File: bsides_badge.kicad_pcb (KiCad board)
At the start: 2 copper layers, 100.5 x 100.5 mm, 2 parts

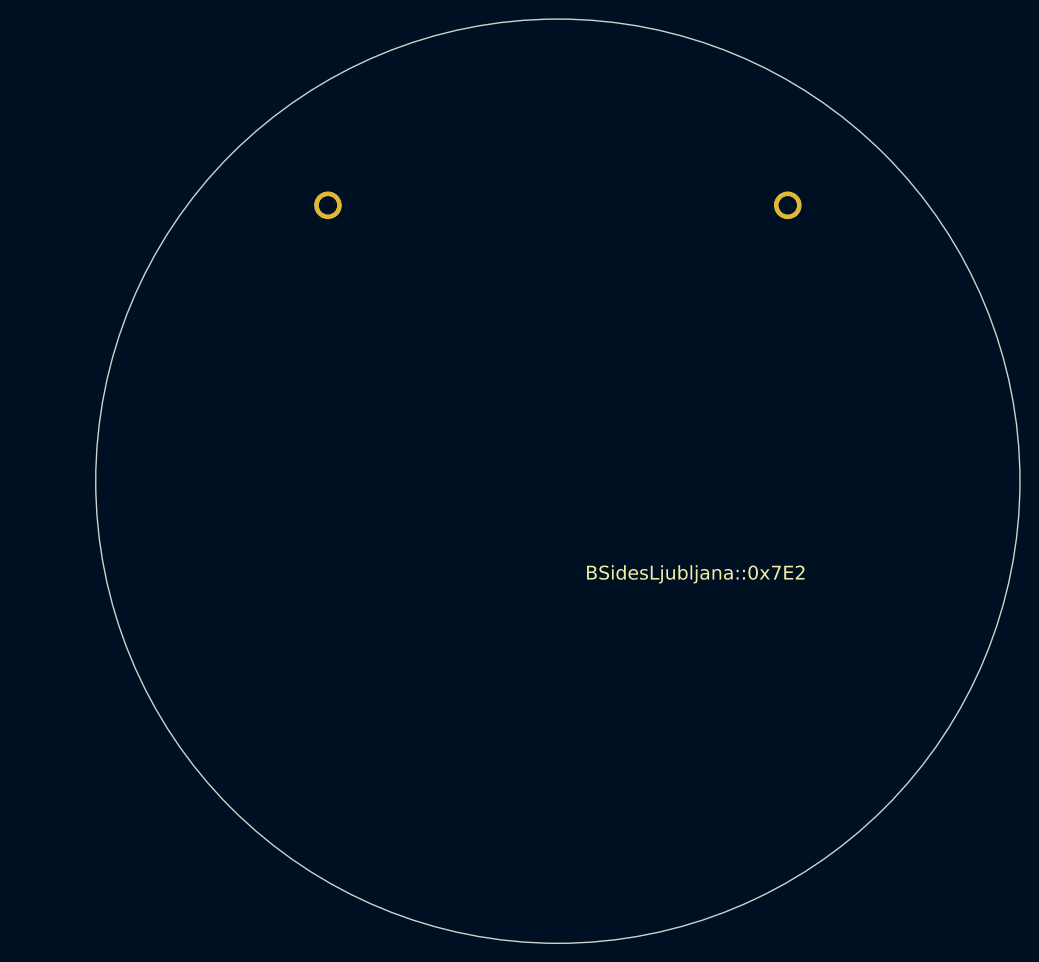
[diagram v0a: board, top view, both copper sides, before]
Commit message: V2 badge
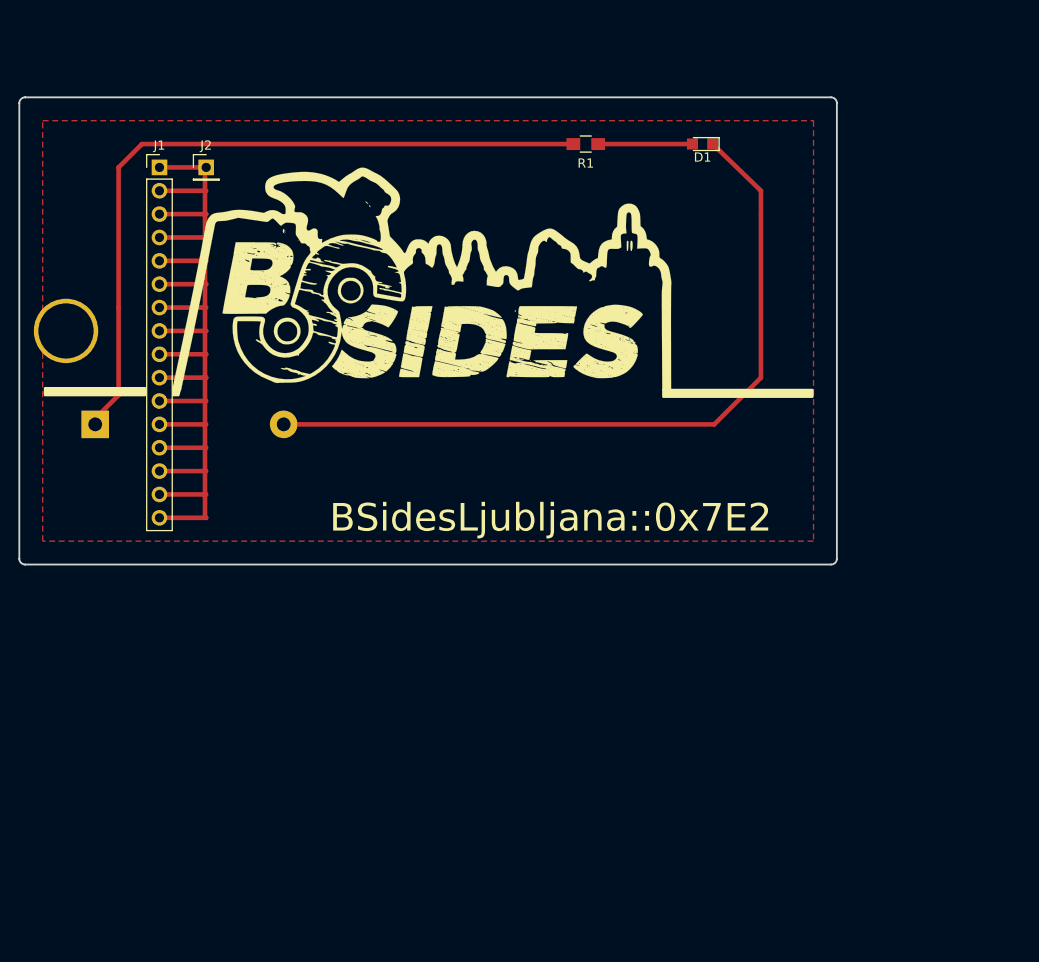
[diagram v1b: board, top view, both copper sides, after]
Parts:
- removed the REF** at (125.0, 60.0)
- removed the REF** at (175.0, 60.0)
- added BT1: Battery_Cell, badge:CoinCell_no_silk, F.Cu at (99.7, 83.8)
- added D1: LED, LEDs:LED_0805, F.Cu at (165.7, 53.3)
- added G***: LOGO, graphics:bsides, F.Cu at (135.6, 68.5)
- added J1: Conn_01x16, Pin_Headers:Pin_Header_Straight_1x16_Pitch2.54mm, F.Cu at (106.7, 55.9)
- added J2: Conn_01x01, Pin_Headers:Pin_Header_Straight_1x01_Pitch2.54mm, F.Cu at (111.8, 55.9)
- added R1: 56R, Resistors_SMD:R_0805_HandSoldering, F.Cu at (153.0, 53.3)
- added REF**: keychain_hole, badge:keychain_hole, F.Cu at (96.5, 73.7)
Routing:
- net Net-(J1-Pad1): track 0.00 -> 120.4 mm
- net Net-(BT1-Pad2): track 0.00 -> 81.6 mm
- net Net-(BT1-Pad1): track 0.00 -> 79.5 mm
- net Net-(D1-Pad2): track 0.00 -> 10.2 mm
- added copper zone on F.Cu, net (none)
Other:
- board size 100.5 x 100.5 mm -> 88.9 x 50.8 mm
- net class Default: clearance 0.2 -> 0.4; trace_width 0.25 -> 0.5
- rule trace_clearance: 0.2 -> 0.4
